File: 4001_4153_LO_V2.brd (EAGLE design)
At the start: 109 x 63 mm, 112 parts, among them IC1 74LVC2G17GV,125, IC10 MCP6H01, IC2 74LVC2G17GV,125, IC3 74LVC2G17GV,125, IC4 ADF4001BRUZ, IC5 ATTINY45V-10SU, IC6 7805DT, IC7 7809DT, IC8 LD1117AS33TR, IC9 ADF4153BRUZ-RL7, Q1 PGA105+

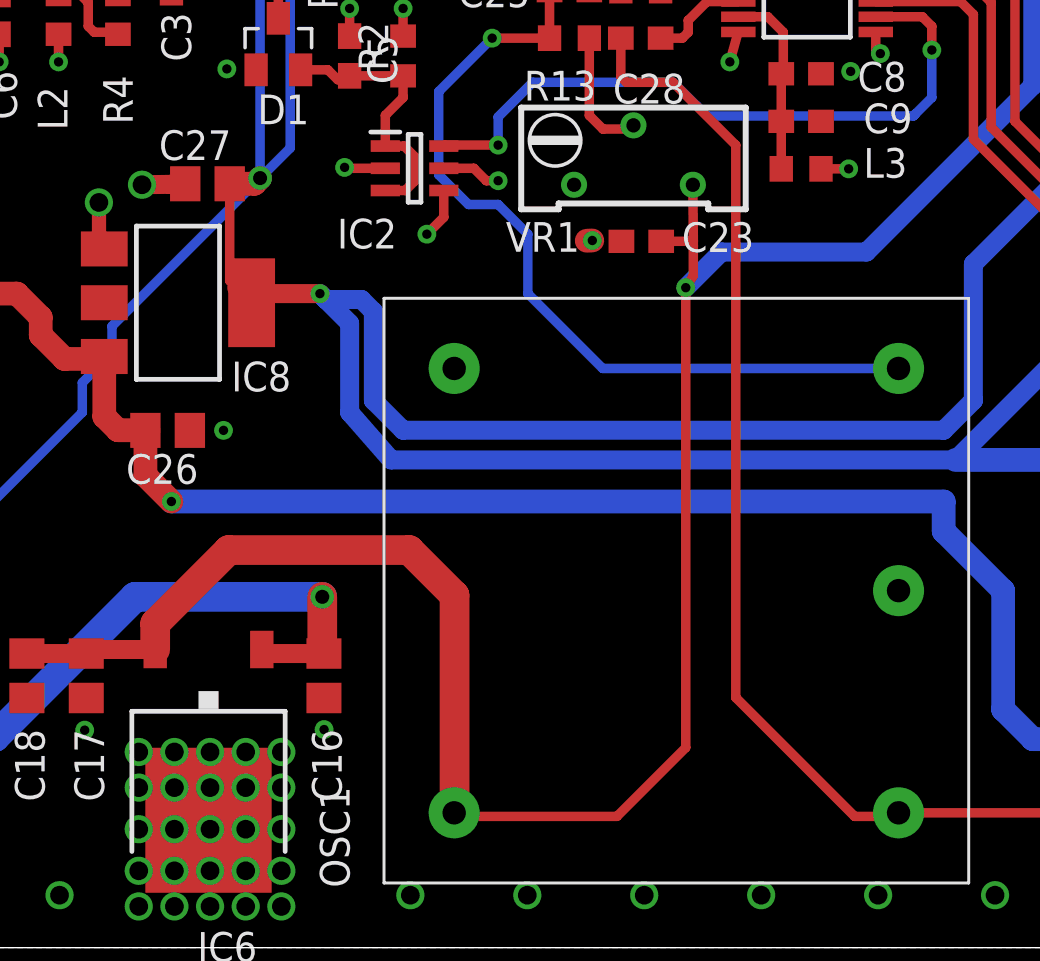
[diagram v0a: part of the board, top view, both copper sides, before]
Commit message: JLC Release
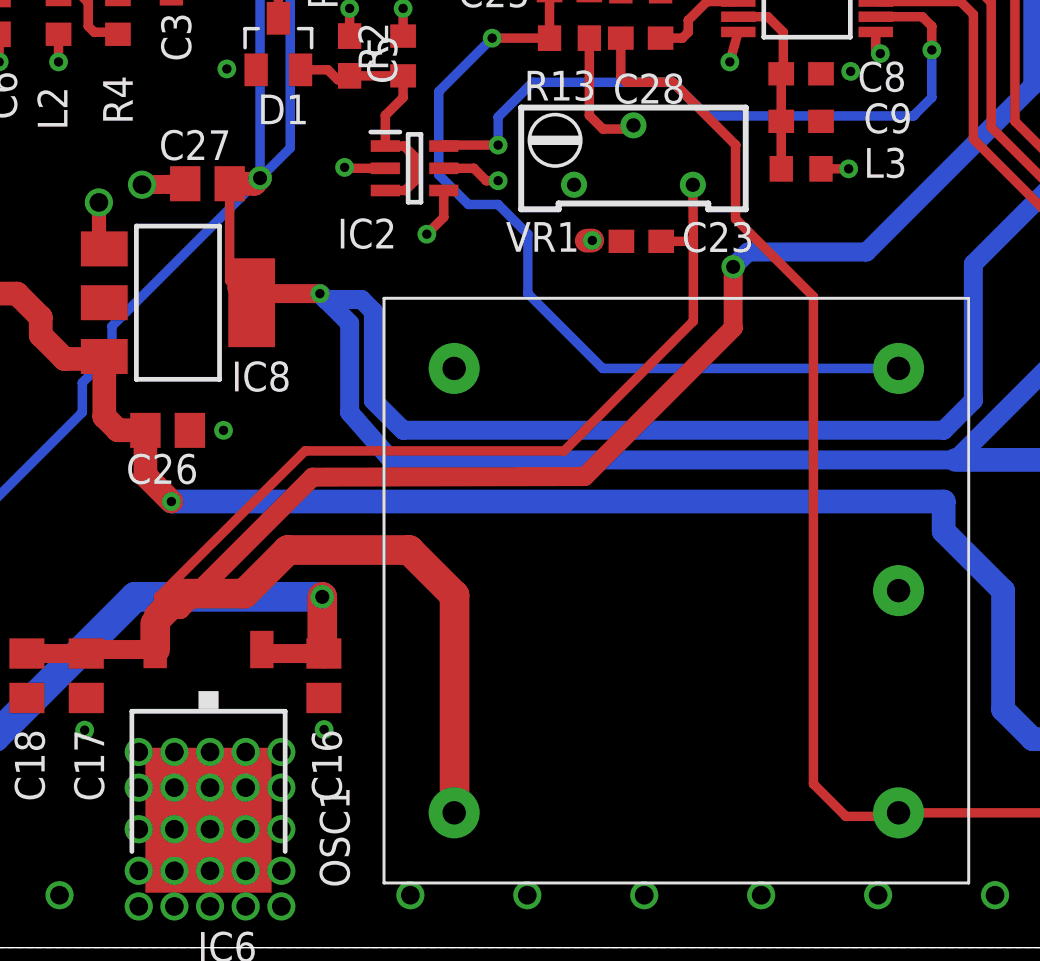
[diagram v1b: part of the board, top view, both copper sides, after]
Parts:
- VR1: value (none) -> 1K0
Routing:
- net +5V: track 128.7 -> 158.1 mm
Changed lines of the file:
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@@
 </element>
 <element name="R29" library="rcl" package="R0603" value="100K" x="34.752" y="42.559" rot="R270"/>
-<element name="VR1" library="resistor" package="RTRIM64Y" value="" x="49.3054" y="32.6186" smashed="yes" rot="R270">
+<element name="VR1" library="resistor" package="RTRIM64Y" value="1K0" x="49.3054" y="32.6186" smashed="yes" rot="R270">
 <attribute name="NAME" x="43.8474" y="29.753" size="1.27" layer="25"/>
 <attribute name="VALUE" x="44.3554" y="29.8686" size="1.27" layer="27"/>
@@
 <contactref element="C23" pad="1"/>
 <contactref element="OSC1" pad="VCC"/>
-<wire x1="51.541759375" y1="28.219" x2="51.541759375" y2="8.554759375" width="0.4064" layer="1"/>
-<wire x1="51.541759375" y1="8.554759375" x2="48.6" y2="5.613" width="0.4064" layer="1"/>
-<wire x1="48.6" y1="5.613" x2="41.792" y2="5.613" width="0.4064" layer="1"/>
 <wire x1="41.792" y1="5.613" x2="41.64" y2="5.765" width="0.4064" layer="1"/>
 <via x="90.3134" y="45.491" extent="1-16" drill="0.4" shape="octagon"/>
@@
 <wire x1="66.38" y1="46.761" x2="66.38" y2="36.855" width="0.8128" layer="16"/>
 <wire x1="66.38" y1="36.855" x2="59.268" y2="29.743" width="0.8128" layer="16"/>
-<wire x1="59.268" y1="29.743" x2="53.065759375" y2="29.743" width="0.8128" layer="16"/>
-<wire x1="53.065759375" y1="29.743" x2="51.541759375" y2="28.219" width="0.8128" layer="16"/>
-<via x="51.541759375" y="28.219" extent="1-16" drill="0.4" shape="octagon"/>
 <contactref element="IC6" pad="2"/>
 <contactref element="C17" pad="1"/>
@@
 <wire x1="41.3" y1="5.425" x2="41.64" y2="5.765" width="0.8128" layer="1"/>
 <wire x1="28.856" y1="12.747" x2="28.856" y2="13.856" width="1.27" layer="1"/>
-<wire x1="28.856" y1="13.856" x2="32" y2="17" width="1.27" layer="1"/>
-<wire x1="32" y1="17" x2="39.7182" y2="17" width="1.27" layer="1"/>
 <wire x1="39.7182" y1="17" x2="41.656" y2="15.0622" width="1.27" layer="1"/>
 <wire x1="41.656" y1="15.0622" x2="41.656" y2="5.781" width="1.27" layer="1"/>
@@
 <wire x1="51.8654" y1="30.2256" x2="51.8454" y2="32.6186" width="0.4064" layer="1"/>
 <wire x1="51.8654" y1="30.2256" x2="51.8654" y2="30" width="0.4064" layer="1"/>
-<wire x1="51.8654" y1="30" x2="51.8654" y2="28.733559375" width="0.4064" layer="1"/>
-<wire x1="51.8654" y1="28.733559375" x2="51.541759375" y2="28.219" width="0.4064" layer="1"/>
 <wire x1="50.4914" y1="30.2002" x2="51.6652" y2="30.2002" width="0.4064" layer="1"/>
 <wire x1="51.6652" y1="30.2002" x2="51.8654" y2="30" width="0.4064" layer="1"/>
+<wire x1="29" y1="15" x2="35.2634" y2="21.238" width="0.4064" layer="1"/>
+<wire x1="35.2634" y1="21.238" x2="46.3426" y2="21.238" width="0.4064" layer="1"/>
+<wire x1="46.3426" y1="21.238" x2="51.8668" y2="26.7876" width="0.4064" layer="1"/>
+<wire x1="51.8668" y1="26.7876" x2="51.8668" y2="29.9986" width="0.4064" layer="1"/>
+<wire x1="51.8668" y1="29.9986" x2="51.8654" y2="30" width="0.4064" layer="1"/>
+<wire x1="59.268" y1="29.743" x2="54.2032" y2="29.743" width="0.8128" layer="16"/>
+<wire x1="54.2032" y1="29.743" x2="53.5686" y2="29.1084" width="0.8128" layer="16"/>
+<via x="53.5686" y="29.1084" extent="1-16" drill="0.6" shape="octagon"/>
+<wire x1="53.5686" y1="29.1084" x2="53.5686" y2="26.4922" width="0.8128" layer="1"/>
+<wire x1="53.5686" y1="26.4922" x2="47.2186" y2="20.1422" width="0.8128" layer="1"/>
+<wire x1="47.2186" y1="20.1422" x2="35.5854" y2="20.1168" width="0.8128" layer="1"/>
+<wire x1="29" y1="15" x2="29" y2="14.1478" width="0.4064" layer="1"/>
+<wire x1="29" y1="14.1478" x2="29" y2="14" width="0.4064" layer="1"/>
+<wire x1="29" y1="14" x2="28.856" y2="13.856" width="0.4064" layer="1"/>
+<wire x1="35.5854" y1="20.1168" x2="29.9212" y2="14.4526" width="0.8128" layer="1"/>
+<wire x1="29.9212" y1="14.4526" x2="29.478" y2="14.478" width="0.8128" layer="1"/>
+<wire x1="29.478" y1="14.478" x2="29" y2="14" width="0.8128" layer="1"/>
+<wire x1="39.7182" y1="17" x2="34.526" y2="17" width="1.27" layer="1"/>
+<wire x1="34.526" y1="17" x2="32.6644" y2="15.1384" width="1.27" layer="1"/>
+<wire x1="32.6644" y1="15.1384" x2="29.9906" y2="15.1384" width="1.27" layer="1"/>
+<wire x1="29.9906" y1="15.1384" x2="29" y2="14.1478" width="1.27" layer="1"/>
 </signal>
 <signal name="OUTPUT">
@@
 <contactref element="C28" pad="2"/>
 <contactref element="OSC1" pad="OUT"/>
-<wire x1="53.68" y1="34.315" x2="53.68" y2="10.693" width="0.4064" layer="1"/>
-<wire x1="53.68" y1="10.693" x2="58.76" y2="5.613" width="0.4064" layer="1"/>
-<wire x1="58.76" y1="5.613" x2="60.488" y2="5.613" width="0.4064" layer="1"/>
+<wire x1="58.387" y1="5.613" x2="60.488" y2="5.613" width="0.4064" layer="1"/>
 <wire x1="60.488" y1="5.613" x2="60.64" y2="5.765" width="0.4064" layer="1"/>
 <wire x1="60.64" y1="5.765" x2="71.104" y2="5.765" width="0.4064" layer="1"/>
@@
 <wire x1="49" y1="37" x2="50.995" y2="37" width="0.4064" layer="1"/>
 <wire x1="50.995" y1="37" x2="53.68" y2="34.315" width="0.4064" layer="1"/>
+<wire x1="58.387" y1="5.613" x2="57" y2="7" width="0.4064" layer="1"/>
+<wire x1="57" y1="7" x2="57" y2="27.836" width="0.4064" layer="1"/>
+<wire x1="57" y1="27.836" x2="53.6702" y2="31.1658" width="0.4064" layer="1"/>
+<wire x1="53.6702" y1="31.1658" x2="53.6702" y2="34.3052" width="0.4064" layer="1"/>
+<wire x1="53.6702" y1="34.3052" x2="53.68" y2="34.315" width="0.4064" layer="1"/>
 </signal>
 <signal name="LE_4153">
@@
 </signal>
 </signals>
-<errors>
-</errors>
 </board>
 </drawing>
